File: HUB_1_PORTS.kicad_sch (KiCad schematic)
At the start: 34 parts, among them U13 VL162, U18 VL162, U20 TPS2560DRCR, U21 TPS2560DRCR

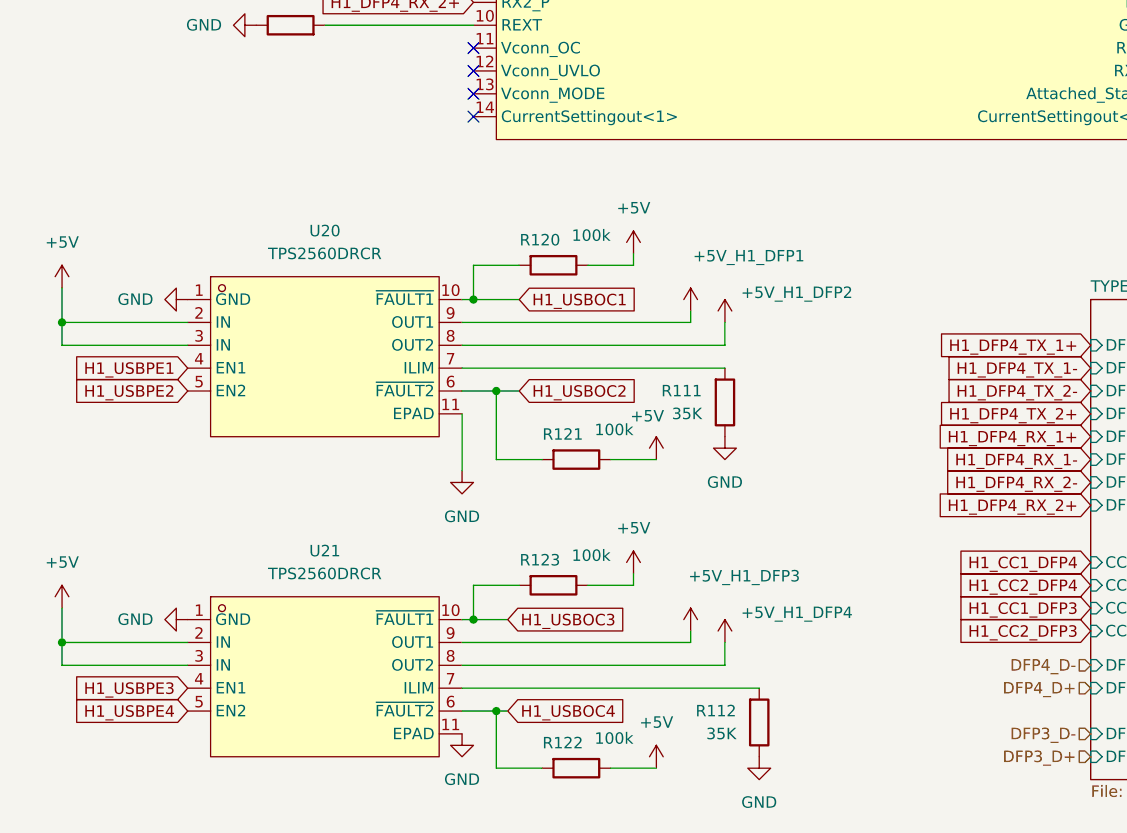
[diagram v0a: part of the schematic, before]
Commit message: .
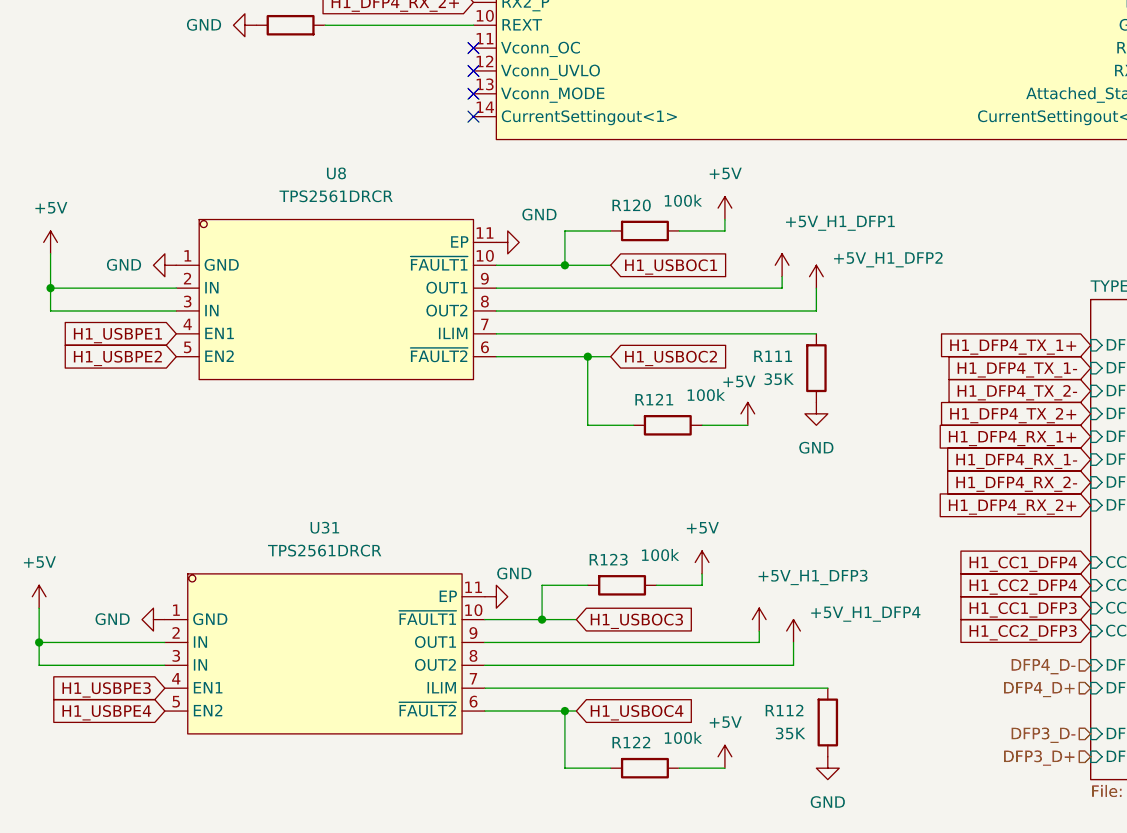
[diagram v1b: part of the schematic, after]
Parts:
- removed U20, U21: TPS2560DRCR, easyeda2kicad:VSON-10_L3.0-W3.0-P0.50-BL-EP_TPS62410DRCR, symbol da:TPS2560DRCR
- added U31, U8: TPS2561DRCR, easyeda2kicad:VSON-10_L3.0-W3.0-P0.50-TL-EP_TPS62410DRCR, symbol da:TPS2561DRCR
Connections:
- net +5V: now also U31.2 (IN), U31.3 (IN), U8.2 (IN), U8.3 (IN)
- net +5V_H1_DFP1: now also U8.9 (OUT1)
- net +5V_H1_DFP2: now also U8.8 (OUT2)
- net +5V_H1_DFP3: now also U31.9 (OUT1)
- net +5V_H1_DFP4: now also U31.8 (OUT2)
- net GND: now also U31.1 (GND), U31.11 (EP), U8.1 (GND), U8.11 (EP)
- net H1_USBOC1: now also U8.10 (~{FAULT1})
- net H1_USBOC2: now also U8.6 (~{FAULT2})
- net H1_USBOC3: now also U31.10 (~{FAULT1})
- net H1_USBOC4: now also U31.6 (~{FAULT2})
- net H1_USBPE1: now also U8.4 (EN1)
- net H1_USBPE2: now also U8.5 (EN2)
- net H1_USBPE3: now also U31.4 (EN1)
- net H1_USBPE4: now also U31.5 (EN2)
- net at R112.2: now also U31.7 (ILIM)
- net at R111.2: now also U8.7 (ILIM)
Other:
- moved on the sheet: R111, R112, R120, R121, R122, R123
